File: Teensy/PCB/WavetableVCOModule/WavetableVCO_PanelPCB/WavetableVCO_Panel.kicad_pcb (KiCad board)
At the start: 2 copper layers, 61 x 128 mm, 15 parts, among them SW1 Next_File_Button

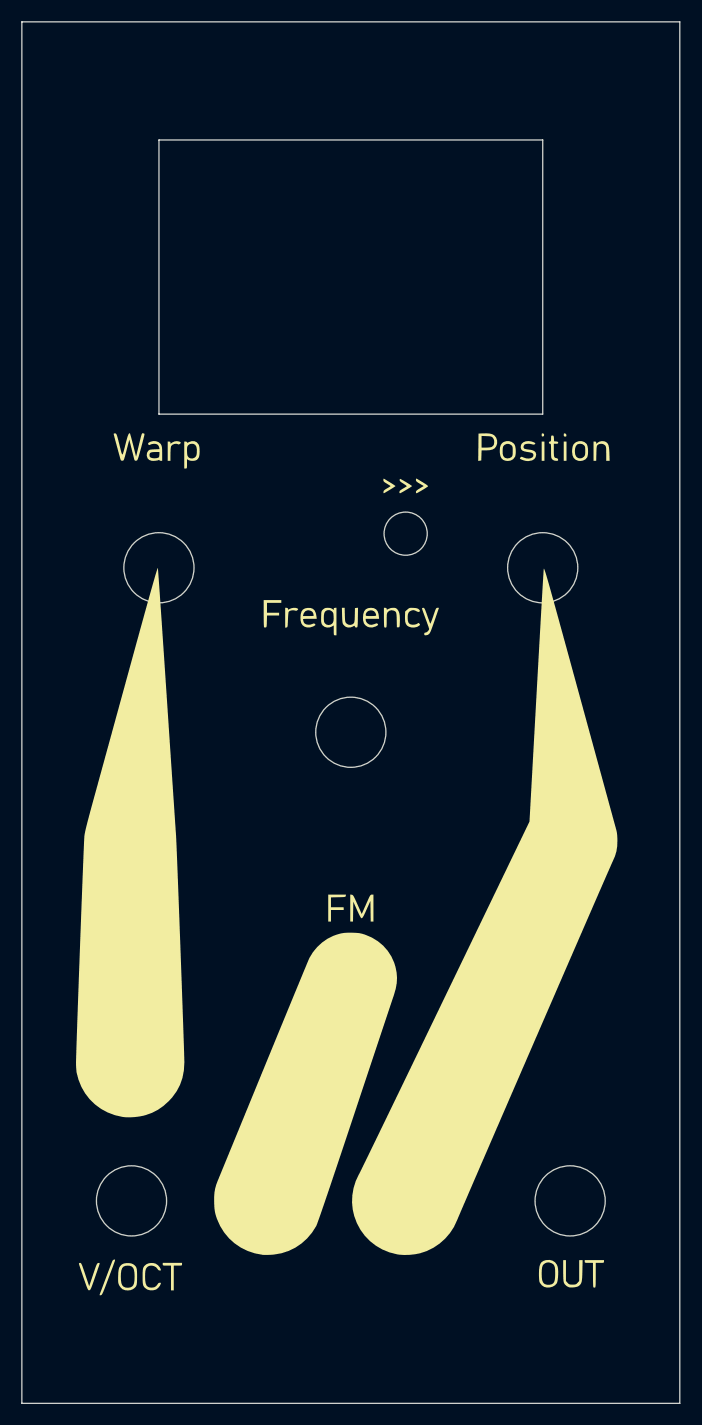
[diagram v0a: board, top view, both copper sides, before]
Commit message: Generated Gerbers
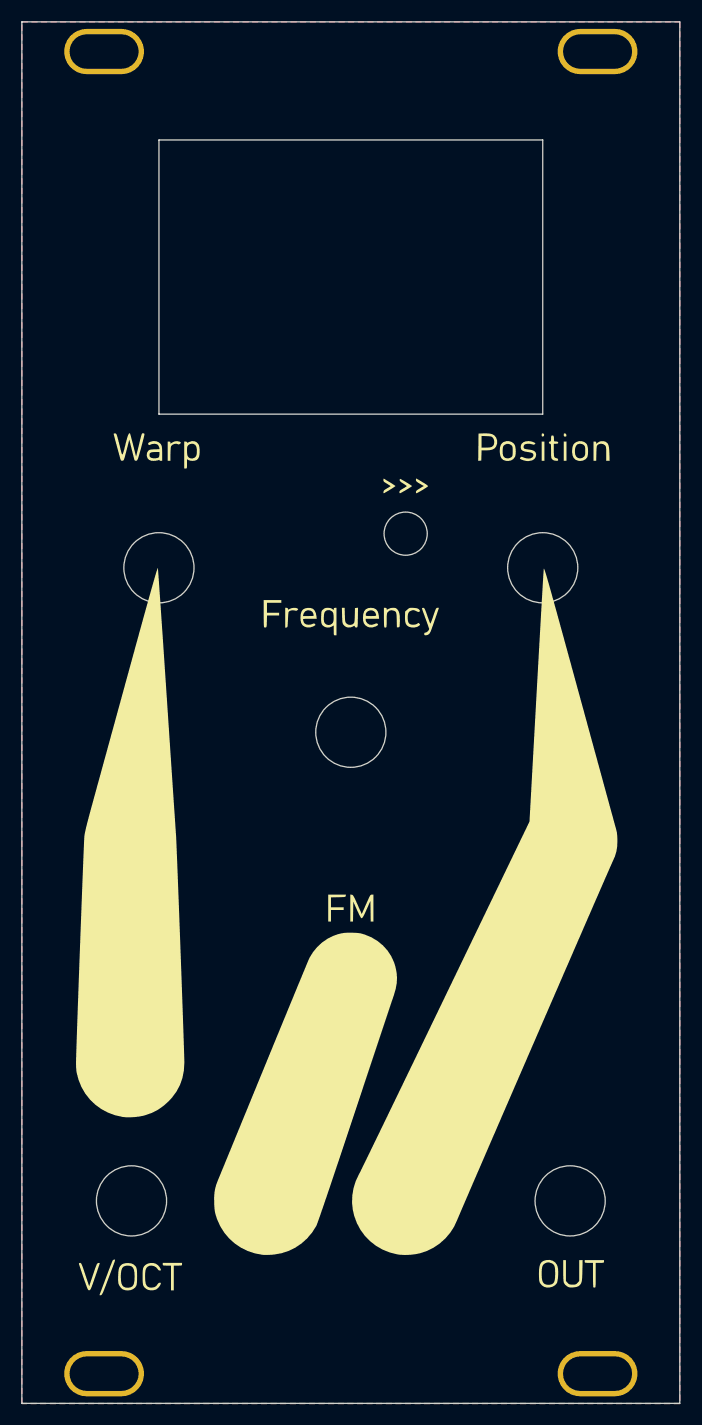
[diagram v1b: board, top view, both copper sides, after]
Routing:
- added copper zone on B.Cu, net extra
- added copper zone on F.Cu, net extra
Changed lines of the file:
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@@
       (layerselection 0x00010fc_ffffffff)
       (disableapertmacros false)
-      (usegerberextensions false)
-      (usegerberattributes true)
-      (usegerberadvancedattributes true)
-      (creategerberjobfile true)
+      (usegerberextensions true)
+      (usegerberattributes false)
+      (usegerberadvancedattributes false)
+      (creategerberjobfile false)
       (svguseinch false)
       (svgprecision 6)
@@
       (psa4output false)
       (plotreference true)
-      (plotvalue true)
+      (plotvalue false)
       (plotinvisibletext false)
       (sketchpadsonfab false)
-      (subtractmaskfromsilk false)
+      (subtractmaskfromsilk true)
       (outputformat 1)
       (mirror false)
-      (drillshape 1)
+      (drillshape 0)
       (scaleselection 1)
-      (outputdirectory "")
+      (outputdirectory "WavetableVCO_Panel_Gerber/")
     )
   )
   (net 0 "")
+  (net 1 "extra")
   (footprint "Perfboard:3.5mm Jack Perfboard_Hole" (layer "F.Cu")
     (at 129.54 154.1)
@@
       (effects (font (size 1 1) (thickness 0.15)))
     )
+    (fp_line (start -2.54 -64) (end 2.54 -64) (layer "User.1") (width 0.12))
     (fp_line (start -2.54 64) (end 2.54 64) (layer "User.1") (width 0.12))
-    (fp_line (start -2.54 -64) (end 2.54 -64) (layer "User.1") (width 0.12))
     (fp_circle (center 0 0) (end 0 0) (layer "User.1") (width 0.12) (fill none))
-    (fp_line (start -1.27 59.65) (end 1.27 59.65) (layer "User.2") (width 0.12))
-    (fp_line (start -1.27 62.85) (end 1.27 62.85) (layer "User.2") (width 0.12))
-    (fp_line (start -1.27 -62.85) (end 1.27 -62.85) (layer "User.2") (width 0.12))
-    (fp_line (start -1.27 -59.65) (end 1.27 -59.65) (layer "User.2") (width 0.12))
-    (fp_arc (start -1.27 62.85) (mid -2.87 61.25) (end -1.27 59.65) (layer "User.2") (width 0.12))
-    (fp_arc (start 1.27 59.65) (mid 2.87 61.25) (end 1.27 62.85) (layer "User.2") (width 0.12))
-    (fp_arc (start -1.27 -59.65) (mid -2.87 -61.25) (end -1.27 -62.85) (layer "User.2") (width 0.12))
-    (fp_arc (start 1.27 -62.85) (mid 2.87 -61.25) (end 1.27 -59.65) (layer "User.2") (width 0.12))
-    (pad "" np_thru_hole oval (at 0 -61.25) (size 5.74 3.2) (drill oval 5.74 3.2) (layers *.Mask))
-    (pad "" np_thru_hole oval (at 0 61.25) (size 5.74 3.2) (drill oval 5.74 3.2) (layers *.Mask))
+    (fp_line (start -1.6 59.65) (end 1.6 59.65) (layer "User.2") (width 0.12))
+    (fp_line (start -1.6 -59.65) (end 1.6 -59.65) (layer "User.2") (width 0.12))
+    (fp_line (start -1.6 62.85) (end 1.6 62.85) (layer "User.2") (width 0.12))
+    (fp_line (start -1.6 -62.85) (end 1.6 -62.85) (layer "User.2") (width 0.12))
+    (fp_arc (start 1.6 59.65) (mid 3.2 61.25) (end 1.6 62.85) (layer "User.2") (width 0.12))
+    (fp_arc (start 1.6 -62.85) (mid 3.2 -61.25) (end 1.6 -59.65) (layer "User.2") (width 0.12))
+    (fp_arc (start -1.6 -59.65) (mid -3.2 -61.25) (end -1.6 -62.85) (layer "User.2") (width 0.12))
+    (fp_arc (start -1.6 62.85) (mid -3.2 61.25) (end -1.6 59.65) (layer "User.2") (width 0.12))
+    (pad "1" thru_hole oval (at 0 -61.25) (size 7.4 4.2) (drill oval 6.4 3.2) (layers *.Cu *.Mask)
+      (net 1 "extra"))
+    (pad "1" thru_hole oval (at 0 61.25) (size 7.4 4.2) (drill oval 6.4 3.2) (layers *.Cu *.Mask)
+      (net 1 "extra"))
   )
   (footprint "Potentiometer:Bourns_PTV09A-XF_Hole" (layer "F.Cu")
@@
     (fp_line (start -2.54 -64) (end 2.54 -64) (layer "User.1") (width 0.12))
     (fp_circle (center 0 0) (end 0 0) (layer "User.1") (width 0.12) (fill none))
-    (fp_line (start -1.27 -59.65) (end 1.27 -59.65) (layer "User.2") (width 0.12))
-    (fp_line (start -1.27 62.85) (end 1.27 62.85) (layer "User.2") (width 0.12))
-    (fp_line (start -1.27 59.65) (end 1.27 59.65) (layer "User.2") (width 0.12))
-    (fp_line (start -1.27 -62.85) (end 1.27 -62.85) (layer "User.2") (width 0.12))
-    (fp_arc (start -1.27 -59.65) (mid -2.87 -61.25) (end -1.27 -62.85) (layer "User.2") (width 0.12))
-    (fp_arc (start -1.27 62.85) (mid -2.87 61.25) (end -1.27 59.65) (layer "User.2") (width 0.12))
-    (fp_arc (start 1.27 -62.85) (mid 2.87 -61.25) (end 1.27 -59.65) (layer "User.2") (width 0.12))
-    (fp_arc (start 1.27 59.65) (mid 2.87 61.25) (end 1.27 62.85) (layer "User.2") (width 0.12))
-    (pad "" np_thru_hole oval (at 0 61.25) (size 5.74 3.2) (drill oval 5.74 3.2) (layers *.Mask))
-    (pad "" np_thru_hole oval (at 0 -61.25) (size 5.74 3.2) (drill oval 5.74 3.2) (layers *.Mask))
+    (fp_line (start -1.6 62.85) (end 1.6 62.85) (layer "User.2") (width 0.12))
+    (fp_line (start -1.6 -62.85) (end 1.6 -62.85) (layer "User.2") (width 0.12))
+    (fp_line (start -1.6 59.65) (end 1.6 59.65) (layer "User.2") (width 0.12))
+    (fp_line (start -1.6 -59.65) (end 1.6 -59.65) (layer "User.2") (width 0.12))
+    (fp_arc (start -1.6 62.85) (mid -3.2 61.25) (end -1.6 59.65) (layer "User.2") (width 0.12))
+    (fp_arc (start 1.6 59.65) (mid 3.2 61.25) (end 1.6 62.85) (layer "User.2") (width 0.12))
+    (fp_arc (start -1.6 -59.65) (mid -3.2 -61.25) (end -1.6 -62.85) (layer "User.2") (width 0.12))
+    (fp_arc (start 1.6 -62.85) (mid 3.2 -61.25) (end 1.6 -59.65) (layer "User.2") (width 0.12))
+    (pad "1" thru_hole oval (at 0 61.25) (size 7.4 4.2) (drill oval 6.4 3.2) (layers *.Cu *.Mask)
+      (net 1 "extra"))
+    (pad "1" thru_hole oval (at 0 -61.25) (size 7.4 4.2) (drill oval 6.4 3.2) (layers *.Cu *.Mask)
+      (net 1 "extra"))
   )
   (footprint "Perfboard:3.5mm Jack Perfboard_Hole" (layer "F.Cu")
@@
   (gr_rect (start 91.442322 56.66449) (end 126.999967 82.065685) (layer "Edge.Cuts") (width 0.05) (fill none))
   (gr_rect (start 78.74 45.72) (end 139.7 173.72) (layer "Edge.Cuts") (width 0.05) (fill none))
+  (zone (net 1) (net_name "extra") (layers F&B.Cu) (hatch edge 0.508)
+    (connect_pads yes (clearance 0.508))
+    (min_thickness 0.254) (filled_areas_thickness no)
+    (fill yes (thermal_gap 0.508) (thermal_bridge_width 0.508))
+    (polygon
+      (pts
+        (xy 139.7 173.736)
+        (xy 78.74 173.736)
+        (xy 78.74 45.72)
+        (xy 139.7 45.72)
+      )
+    )
+  )
 )
